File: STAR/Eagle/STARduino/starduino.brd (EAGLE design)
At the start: 59.7 x 38.2 mm, 73 parts, among them J1 J30J-25, U1 SSCMNNN015PA2A3, U10 MC14504BDTG, U11 MAX31725MTA+, U12 TCA9535_RTW_24, U13 BMX055, U15 MC74VHC1GT125, U16 PCA9515A, U17 PCA9306DCT, U18 LT8616, U4 DS3231MZ+, U6 ATSAMD21G18, U8 ADXL375BCCZ

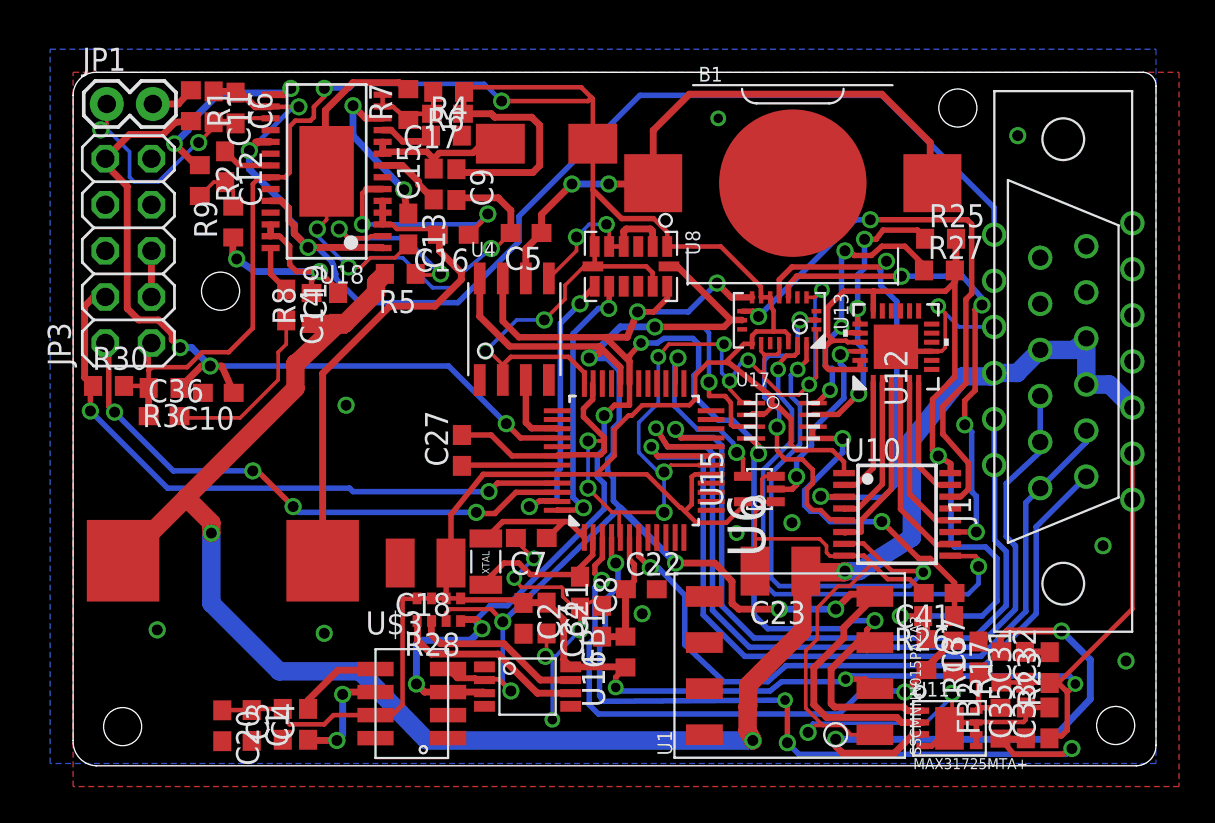
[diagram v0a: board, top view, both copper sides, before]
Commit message: misc board stuff
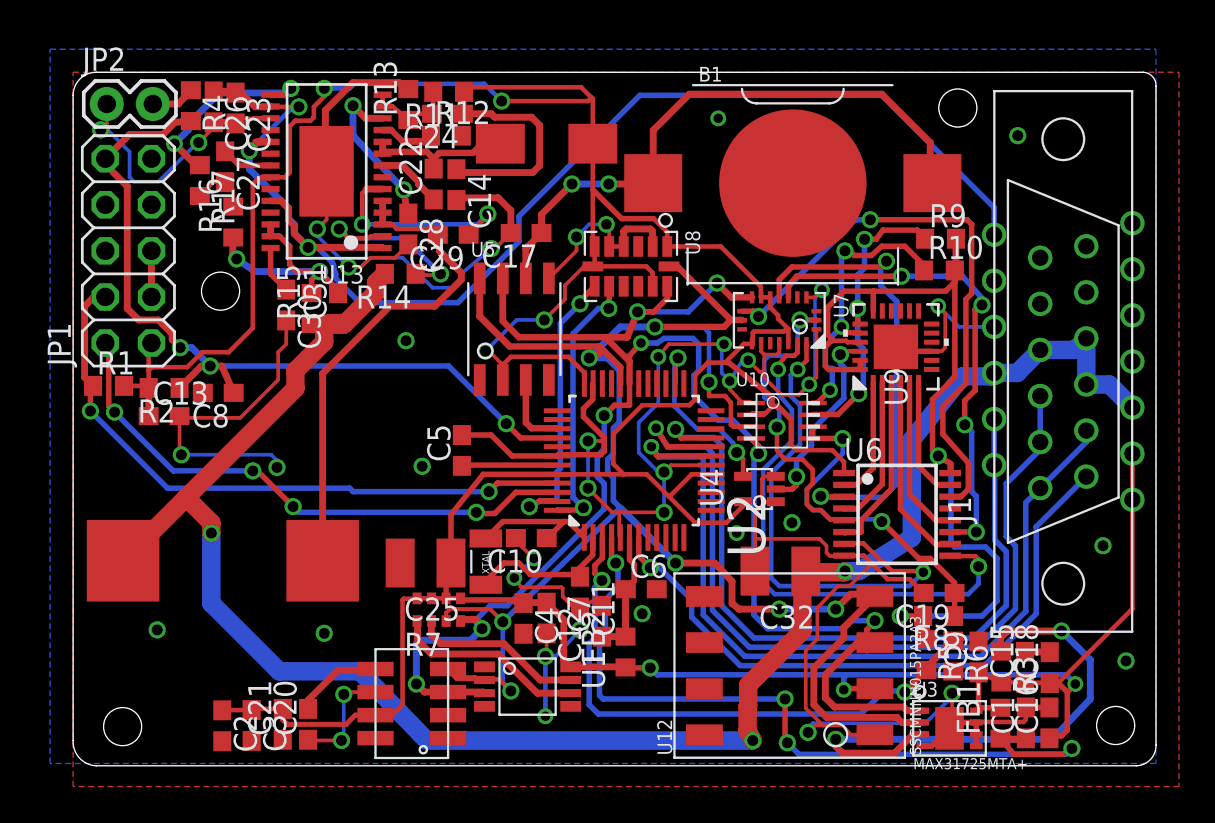
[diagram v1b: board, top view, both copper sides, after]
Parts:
- removed C33, C34, C35, C36, C37: 100nF, resistor:C0603
- removed C41: 100pF, rcl:C0603
- removed JP3: (no value), pinhead:2X05
- removed R23: 4.7k, resistor:R0603
- removed R25: 4.7k, rcl:R0603
- removed R26: 220k, rcl:R0603
- removed R28: 4.7k, SparkFun-Passives:0603-ARV
- removed R30: 10k, resistor:R0603
- removed U$3: CC2, NR_IC:CC2
- removed U15: MC74VHC1GT125, CM_IC:SC-70-5
- removed U16: PCA9515A, CM_IC:TSSOP8
- removed U17: PCA9306DCT, MotorDriver:SSOP8
- removed U18: LT8616, AR_IC:28-TSSOP
- added C24: 4.7pF, rcl:C0603
- added C25: 47uF, resistor:C1210
- added C26: 4.7uF, resistor:C0603
- added C28, C30: 1nF, resistor:C0603
- added C29: 100nF, resistor:C0603
- added JP2: (no value), CM_passives:1X02
- added R11: 560k, resistor:R0603
- added R12, R14: 1M, resistor:R0603
- added R13: 176k, resistor:R0603
- added R15: 820k, resistor:R0603
- added U2: ATSAMD21G18, AR_mcu:48-TQFP
- added U3: MAX31725MTA+, NR_IC:DFN-8
- added U5: DS3231MZ+, NR_IC:SOIC-8
- added U7: BMX055, NR_IC:LGA-20
- added U9: TCA9535_RTW_24, MotorDriver:RTW24_2P45X2P45
- C10: value 100nF -> 6.8pF
- C11: value 4.7uF -> 6.8pF
- C12: value 1uF -> 100nF
- C13, C14: value 1nF -> 100nF
- C15: value 100nF -> 10uF
- C17: value 4.7pF -> 1nF; device rcl:C0603 -> resistor:C0603
- C18: value 47uF -> 100nF; device resistor:C1210 -> resistor:C0603
- C19: value 4.7pF -> 100pF
- C21: value 100nF -> 220nF
- C22: value 10uF -> 100nF
- C23: value 47uF -> 4.7uF; device resistor:C1210 -> resistor:C0603
- C3: value 220nF -> 100nF
- C31: value 10uF -> 4.7pF; device resistor:C0603 -> rcl:C0603
- C32: value 100nF -> 47uF; device resistor:C0603 -> resistor:C1210
- C5: value 1nF -> 1uF
- C6: value 4.7uF -> 10uF
- C7, C8: value 6.8pF -> 100nF
- JP1: device CM_passives:1X02 -> pinhead:2X05
- R1: value 330 -> 10k
- R16: value 3.6k -> 154k
- R17: value 6.8k -> 24.3k
- R2: value 24.3k -> 10k
- R3: value 10k -> 4.7k
- R4: value 1M -> 330
- R5: value 1M -> 3.6k
- R6: value 560k -> 6.8k
- R7: value 176k -> 4.7k; device resistor:R0603 -> SparkFun-Passives:0603-ARV
- R8: value 820k -> 220k; device resistor:R0603 -> rcl:R0603
- R9: value 154k -> 4.7k; device resistor:R0603 -> rcl:R0603
- U1: value SSCMNNN015PA2A3 -> PCA9515A; device NR_IC:HSC-SMT-8 -> CM_IC:TSSOP8
- U10: value MC14504BDTG -> PCA9306DCT; device MotorDriver:TSSOP16 -> MotorDriver:SSOP8
- U11: value MAX31725MTA+ -> CC2; device NR_IC:DFN-8 -> NR_IC:CC2
- U12: value TCA9535_RTW_24 -> SSCMNNN015PA2A3; device MotorDriver:RTW24_2P45X2P45 -> NR_IC:HSC-SMT-8
- U13: value BMX055 -> LT8616; device NR_IC:LGA-20 -> AR_IC:28-TSSOP
- U4: value DS3231MZ+ -> MC74VHC1GT125; device NR_IC:SOIC-8 -> CM_IC:SC-70-5
- U6: value ATSAMD21G18 -> MC14504BDTG; device AR_mcu:48-TQFP -> MotorDriver:TSSOP16
- moved R17 49.1 mm to (6.99, 32.1)
- moved R3 48.6 mm to (51.2, 5.32), turned to 270 degrees
- moved R16 45.0 mm to (8.83, 29.8), turned to 90 degrees
- moved C31 42.7 mm to (14.6, 25.1)
- moved C1 42.7 mm to (52.5, 2.24), turned to 90 degrees
- moved C16 42.5 mm to (53.8, 2.24), turned to 90 degrees
- moved C15 42.1 mm to (52.5, 5.30)
- moved R6 41.7 mm to (48.5, 5.92), turned to 270 degrees
- moved C23 39.4 mm to (8.95, 36.1), turned to 270 degrees
- moved R9 39.0 mm to (47.8, 28.9), turned to 0 degrees
- moved C9 38.8 mm to (49.9, 5.87), turned to 90 degrees
- moved R8 38.5 mm to (47.7, 8.13), turned to 180 degrees
- moved C19 36.7 mm to (47.7, 9.40), turned to 180 degrees
- moved R5 35.8 mm to (47.0, 6.00), turned to 270 degrees
- moved C18 34.9 mm to (53.8, 5.29), turned to 90 degrees
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- renumbered R27 to R10, U$1 to IMAG2, U$2 to IMAG1
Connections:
- net +3V3: now also C12.1, C13.1, C14.1, C15.1, C16.1, C21.2, C24.1, C25.1, C3.1, C4.1, FB1.2, FB2.1, JP1.1, R1.2, R11.1, R12.2, R2.2, R7.5, R7.6, R7.7, R7.8, U1.P$8, U10.2, U11.P$7, U12.2, U13.22, U2.17, U2.36, U2.44, U3.8, U4.5, U5.2, U6.1, U7.12, U7.13, U7.3, U7.7; no longer C1.1, C17.1, C20.1, C3.2, C31.1, C32.1, C33.1, C34.1, C36.1, C37.1, FB1.1, FB2.2, JP3.1, R23.2, R28.5, R28.6, R28.7, R28.8, R30.2, R4.2, R6.1, U$3.P$7, U1.2, U10.1, U11.8, U13.12, U13.13, U13.3, U13.7, U15.5, U16.P$8, U17.2, U18.22, U4.2, U6.17, U6.36, U6.44
- net +5V: now also C31.1, C32.1, R14.2, R15.1; no longer C19.1, C23.1, R5.2, R8.1
- net 5V_S: now also R5.1, R8.2, R9.2, U6.16, U9.18, U9.21, U9.23, U9.24; no longer R16.1, R25.2, R26.2, U10.16, U12.18, U12.21, U12.23, U12.24
- net BIAS_REF: now also U2.7; no longer U6.7
- net DEC0: now also U9.15; no longer U12.15
- net DEC1: now also U9.13; no longer U12.13
- net DIR: now also U9.12; no longer U12.12
- net EN_28V: now also U2.41; no longer U6.41
- net GND: now also C15.2, C16.2, C17.2, C19.2, C20.1, C21.1, C25.2, C26.2, C28.2, C3.2, C30.2, C4.2, JP1.3, JP1.5, JP2.1, R13.2, R16.2, R6.2, U1.P$4, U10.1, U11.P$6, U12.1, U13.29, U2.18, U2.35, U2.42, U2.5, U3.4, U3.5, U3.6, U3.7, U3.9, U4.1, U4.3, U5.5, U6.13, U6.8, U7.17, U7.20, U7.4, U7.6, U9.25, U9.9; no longer C20.2, C21.2, C22.2, C3.1, C31.2, C33.2, C34.2, C35.2, C36.2, C37.2, C4.1, C41.2, JP1.1, JP3.3, JP3.5, R2.2, R7.2, R9.2, U$3.P$6, U1.1, U10.13, U10.8, U11.4, U11.5, U11.6, U11.7, U11.9, U12.25, U12.9, U13.20, U13.4, U13.6, U15.1, U15.3, U16.P$4, U17.1, U18.17, U18.29, U4.5, U6.18, U6.35, U6.42, U6.5
- net I0: now also U9.17; no longer U12.17
- net I1: now also U9.16; no longer U12.16
- net IMUDR: now also U6.9, U7.2; no longer U10.9, U13.2
- net IMUINT1: now also U6.5, U7.19; no longer U10.5, U13.19
- net IMUINT2: now also U6.7, U7.1; no longer U10.7, U13.1
- net IMUINT3: now also U6.3, U7.14; no longer U10.3, U13.14
- net IMUINT4: now also U6.11, U7.15; no longer U10.11, U13.15
- net IMUINT5: now also U6.14, U7.10; no longer U10.14, U13.10
- net IOEINT: now also U2.26, U4.4; no longer U15.4, U6.26
- net I_SENSE: now also U2.10; no longer U6.10
- net LED_CTRL: now also U2.14; no longer U6.14
- net M0: now also U9.11; no longer U12.11
- net M1: now also U9.10; no longer U12.10
- net MISO: now also U2.21; no longer U6.21
- net MOSI: now also U2.19; no longer U6.19
- net N$1: now also R17.1, U13.15; no longer R2.1, U18.15
- net N$10: now also C6.1, C7.1, FB2.2, U2.6; no longer C21.1, C22.1, FB1.2, U6.6
- net N$11: now also C29.1, U13.6; no longer C16.1, U18.6
- net N$12: now also C22.1, U13.8; no longer C15.1, U18.8
- net N$14: now also C22.2, U13.10, U13.9; no longer C15.2, U18.10, U18.9
- net N$17: now also C29.2, U13.3, U13.4, U13.5; no longer C16.2, U18.3, U18.4, U18.5
- net N$19: now also U6.2, U9.1; no longer U10.2, U12.1
- net N$2: now also C20.2, U11.P$5; no longer C4.2, U$3.P$5
- net N$20: now also R12.1, U13.11; no longer R4.1, U18.11
- net N$21: now also R14.1, U13.2; no longer R5.1, U18.2
- net N$22: now also C24.2, R11.2, R13.1, U13.13, U13.14; no longer C17.2, R6.2, R7.1, U18.13, U18.14
- net N$23: now also U6.4, U9.2; no longer U10.4, U12.2
- net N$25: now also U4.2, U9.22; no longer U12.22, U15.2
- net N$28: now also U6.6, U9.3; no longer U10.6, U12.3
- net N$29: now also U6.10, U9.4; no longer U10.10, U12.4
- net N$3: now also C27.1, U13.21; no longer C12.1, U18.21
- net N$30: now also U6.12, U9.5; no longer U10.12, U12.5
- net N$31: now also U6.15, U9.6; no longer U10.15, U12.6
- net N$33: now also U10.8, U9.20; no longer U12.20, U17.8
- net N$34: now also R9.1, U10.7, U9.19; no longer R25.1, U12.19, U17.7
- net N$35: now also C19.1, R8.1, U10.5, U10.6; no longer C41.1, R26.1, U17.5, U17.6
- net N$37: now also C31.2, R15.2, R16.1, U13.26, U13.27; no longer C19.2, R8.2, R9.1, U18.26, U18.27
- net N$4: now also C28.1, U13.12; no longer C13.1, U18.12
- net N$5: now also C5.1, U2.43; no longer C27.1, U6.43
- net N$6: now also R3.1, U3.3; no longer R23.1, U11.3
- net N$7: now also JP2.2, R4.1; no longer JP1.2, R1.1
- net N$8: now also C17.1, U5.6; no longer C5.1, U4.6
- net N$9: now also C30.1, U13.28; no longer C14.1, U18.28
- net NENBL: now also U9.8; no longer U12.8
- net NFAULT: now also U9.7; no longer U12.7
- net NSLEEP: now also U9.14; no longer U12.14
- net PA27: now also U2.39, U5.3; no longer U4.3, U6.39
- net PB02: now also U2.47; no longer U6.47
- net PB03: now also U2.48; no longer U6.48
- net PB22: now also U2.37; no longer U6.37
- net PB23: now also U2.38; no longer U6.38
- net PI_KILL: now also U2.25; no longer U6.25
- net RESET: now also C8.1, JP1.10, R2.1, R4.2, U2.40; no longer C10.1, JP3.10, R1.2, R3.1, U6.40
- net RX0: now also U2.16; no longer U6.16
- net RX1: now also U2.28; no longer U6.28
- net RX2: now also U2.30; no longer U6.30
- net SCK: now also U2.20; no longer U6.20
- net SCL: now also R7.3, U1.P$2, U10.3, U11.P$4, U12.4, U2.32, U3.2, U5.8, U7.9; no longer R28.3, U$3.P$4, U1.4, U11.2, U13.9, U16.P$2, U17.3, U4.8, U6.32
- net SCL_BUFF: now also R7.2, U1.P$7; no longer R28.2, U16.P$7
- net SDA: now also R7.4, U1.P$3, U10.4, U11.P$3, U12.3, U2.31, U3.1, U5.7, U7.11; no longer R28.4, U$3.P$3, U1.3, U11.1, U13.11, U16.P$3, U17.4, U4.7, U6.31
- net SDA_BUFF: now also R7.1, U1.P$6; no longer R28.1, U16.P$6
- net STEPFREQ: now also U2.13; no longer U6.13
- net SWDCLK: now also JP1.4, R1.1, U2.45; no longer JP3.4, R30.1, U6.45
- net SWDIO: now also JP1.2, U2.46; no longer JP3.2, U6.46
- net SYNC: now also U2.24; no longer U6.24
- net TX0: now also U2.15; no longer U6.15
- net TX1: now also U2.27; no longer U6.27
- net TX2: now also U2.29; no longer U6.29
- net USB_D_N: now also U2.33; no longer U6.33
- net USB_D_P: now also U2.34; no longer U6.34
- net VDD: now also C23.1, C26.1, U13.1, U13.16, U13.19, U13.24; no longer C11.1, C6.1, U18.1, U18.16, U18.19, U18.24
- net VREFA: now also C1.1, FB1.1, U2.4; no longer C35.1, FB2.1, U6.4
- net V_SENSE: now also R5.2, R6.1, U2.3; no longer R16.2, R17.1, U6.3
- net XIN32: now also C10.1, U2.1; no longer C7.1, U6.1
- net XOUT32: now also C11.1, U2.2; no longer C8.1, U6.2
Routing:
- net GND: track 231.6 -> 239.5 mm, vias 37 -> 40
- net BIAS_REF: track 37.6 -> 35.8 mm
- net +3V3: track 252.7 -> 251.4 mm
